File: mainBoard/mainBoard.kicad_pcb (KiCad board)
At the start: 4 copper layers, 50 x 60 mm, 46 parts, among them J1 Conn_01x04, J10 Conn_02x07_Odd_Even, J2 Conn_01x04, J3 Conn_01x03, J6 Conn_01x07, J7 Conn_01x07, J8 Conn_01x02, M1 Conn_01x01, M2 Conn_01x01, U1 MAX15062A, U2 STM32H503CBT6, U3 DRV8251ADDAR

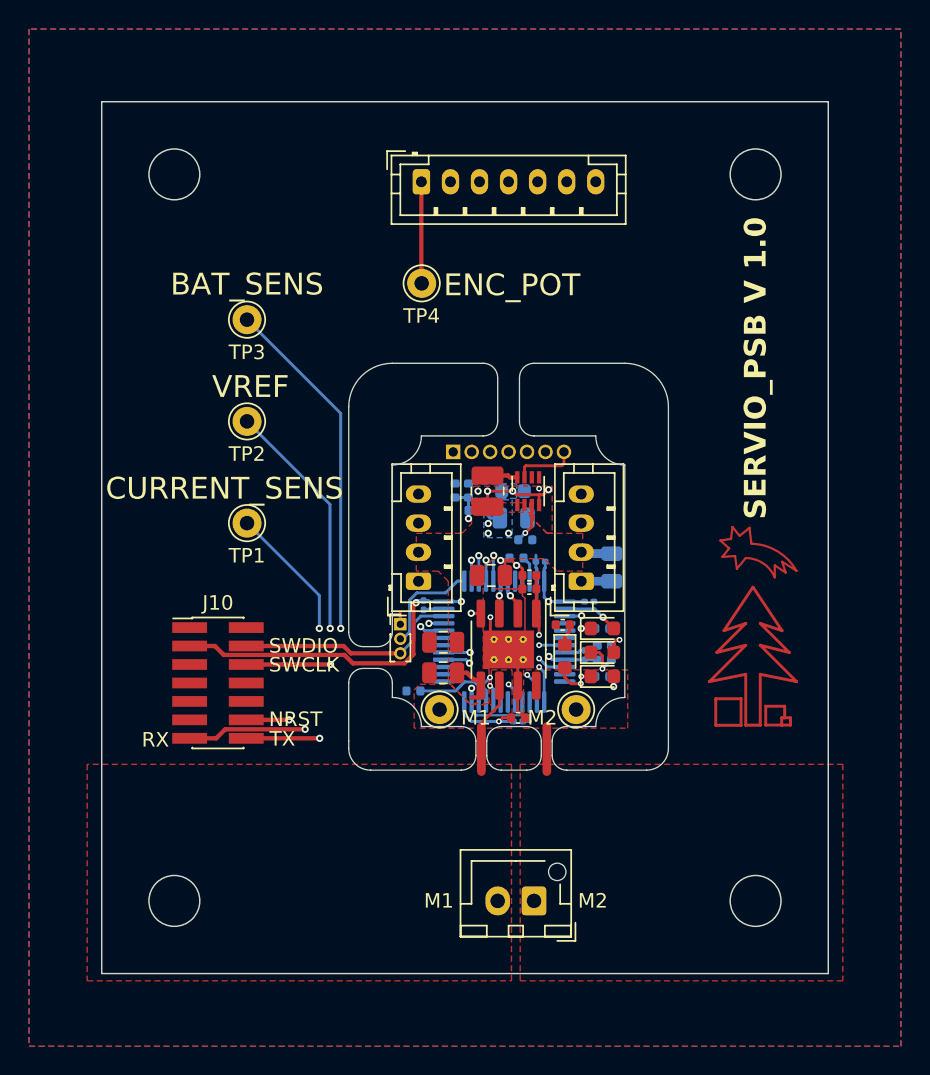
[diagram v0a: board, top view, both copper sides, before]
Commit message: drobeček
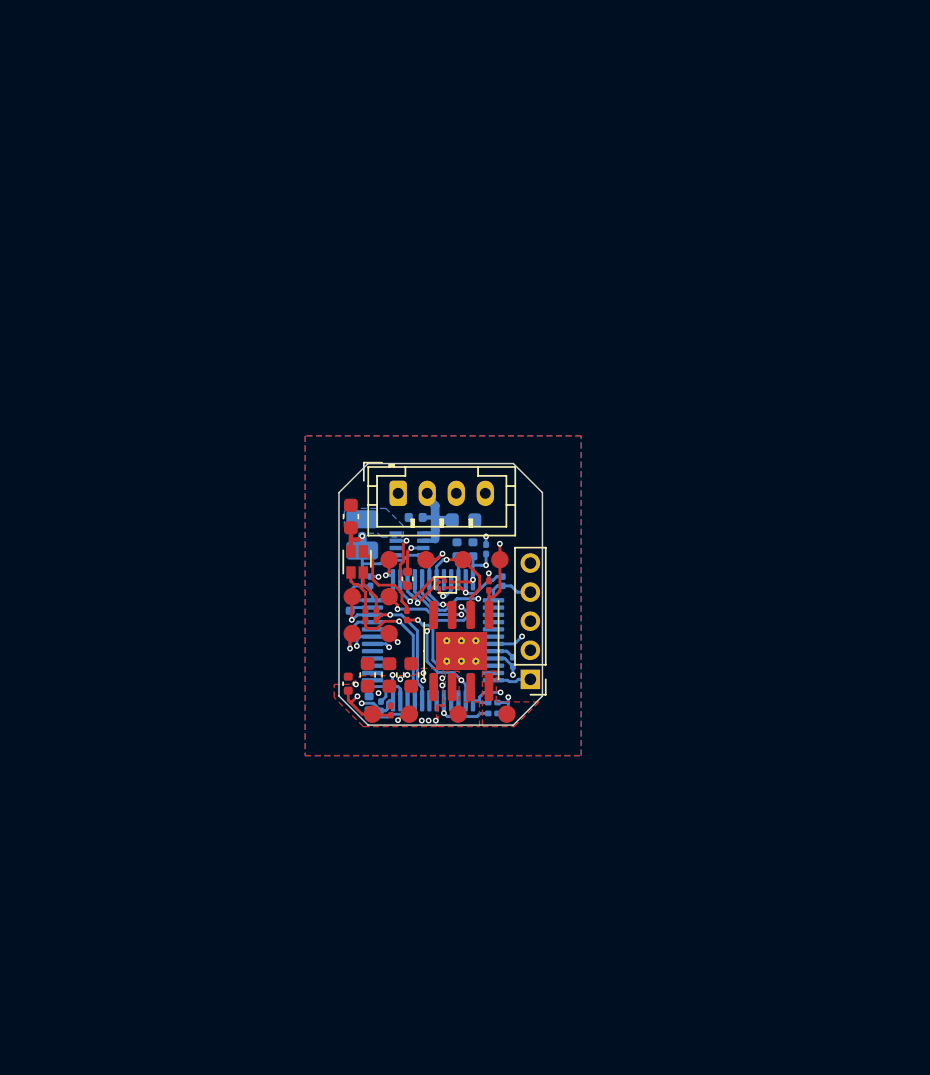
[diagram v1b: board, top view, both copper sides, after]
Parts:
- removed D1: LED-R, LED_SMD:LED_0603_1608Metric
- removed D2: LED-G, LED_SMD:LED_0603_1608Metric
- removed D3: LED-B, LED_SMD:LED_0603_1608Metric
- removed D4: LED-Y, LED_SMD:LED_0603_1608Metric
- removed R3: 1k, Capacitor_SMD:C_0402_1005Metric
- removed TP1, TP2, TP3, TP4: Conn_01x01, Connector_Pin:Pin_D1.0mm_L10.0mm
- added D5: LED_RGAB, LED_SMD:LED_LiteOn_LTST-C19HE1WT, F.Cu at (142.6, 96.7)
- added J11: Conn_01x01, RKL-Connectors:YZ157015035P-01-contact_pad, F.Cu at (144.8, 99.1)
- added J12: Conn_01x01, RKL-Connectors:YZ157015035P-01-contact_pad, F.Cu at (142.2, 101.6)
- added J13: Conn_01x01, RKL-Connectors:YZ157015035P-01-contact_pad, F.Cu at (144.8, 101.6)
- added J4: Conn_01x01, RKL-Connectors:YZ157015035P-01-contact_pad, F.Cu at (146.2, 107.2)
- added J9: Conn_01x01, RKL-Connectors:YZ157015035P-01-contact_pad, F.Cu at (142.2, 99.1)
- added U4: 64Kbit, RKL-StandardPackages:XFBGA-6, F.Cu at (148.7, 98.2)
- C1, C3, C4: moved to F.Cu
- C14: footprint Capacitor_SMD:C_0805_2012Metric -> Capacitor_SMD:C_0603_1608Metric; moved to F.Cu
- C15, R6: footprint Capacitor_SMD:C_0402_1005Metric -> Capacitor_SMD:C_0201_0603Metric
- C16, C17: footprint Capacitor_SMD:C_0805_2012Metric -> Capacitor_SMD:C_0603_1608Metric
- C18: footprint Capacitor_SMD:C_0805_2012Metric -> Capacitor_SMD:C_0603_1608Metric; moved to B.Cu
- C2: footprint Capacitor_SMD:C_0805_2012Metric -> Capacitor_SMD:C_0402_1005Metric
- C5, L1, U1: moved to B.Cu
- J10: value Conn_02x07_Odd_Even -> Conn_01x01; footprint Connector_PinHeader_1.27mm:PinHeader_2x07_P1.27mm_Vertical_SMD -> RKL-Connectors:YZ157015035P-01-contact_pad
- J2: value Conn_01x04 -> Conn_01x01; footprint Connector_JST:JST_PH_B4B-PH-K_1x04_P2.00mm_Vertical -> RKL-Connectors:YZ157015035P-01-contact_pad
- J3: value Conn_01x03 -> Conn_01x01; footprint Connector_PinHeader_1.00mm:PinHeader_1x03_P1.00mm_Vertical -> RKL-Connectors:YZ157015035P-01-contact_pad
- J6: value Conn_01x07 -> Conn_01x01; footprint Connector_JST:JST_PH_B7B-PH-K_1x07_P2.00mm_Vertical -> RKL-Connectors:YZ157015035P-01-contact_pad
- J7: value Conn_01x07 -> Conn_01x05; footprint Connector_PinHeader_1.27mm:PinHeader_1x07_P1.27mm_Vertical -> Connector_PinHeader_2.00mm:PinHeader_1x05_P2.00mm_Vertical; moved to F.Cu
- J8: value Conn_01x02 -> Conn_01x01; footprint Connector_JST:JST_XH_B2B-XH-AM_1x02_P2.50mm_Vertical -> RKL-Connectors:YZ157015035P-01-contact_pad
- M1, M2: footprint Connector_Pin:Pin_D1.0mm_L10.0mm -> RKL-Connectors:YZ157015035P-01-contact_pad
- R1: footprint Capacitor_SMD:C_0402_1005Metric -> Resistor_SMD:R_0201_0603Metric; moved to F.Cu
- R2: footprint Capacitor_SMD:C_0402_1005Metric -> Resistor_SMD:R_0201_0603Metric
- R4, R5: footprint Capacitor_SMD:C_0402_1005Metric -> Capacitor_SMD:C_0201_0603Metric; moved to F.Cu
- R7: footprint Capacitor_SMD:C_0402_1005Metric -> Capacitor_SMD:C_0201_0603Metric; moved to B.Cu
- moved J6 26.0 mm to (147.3, 96.5)
- moved J8 24.0 mm to (149.9, 96.5), turned to 0 degrees
- moved J2 17.0 mm to (143.6, 107.2), turned to 0 degrees
- moved R4 16.8 mm to (143.2, 100.3), turned to -90 degrees
- moved J7 16.5 mm to (154.5, 104.8), turned to 180 degrees
- moved R5 16.4 mm to (143.9, 100.3), turned to -90 degrees
- moved C14 15.7 mm to (146.3, 104.5), turned to 90 degrees
- moved C1 15.7 mm to (142.0, 105.0)
- moved R2 15.6 mm to (151.9, 107.1), turned to 180 degrees
- moved C6 15.1 mm to (143.5, 98.0), turned to 90 degrees
- moved R1 14.9 mm to (144.9, 106.9), turned to -90 degrees
- moved J10 14.5 mm to (144.8, 96.5)
- moved C10 14.5 mm to (144.2, 106.6)
- moved C5 14.0 mm to (142.1, 99.5), turned to -90 degrees
- moved C7 12.1 mm to (151.4, 95.8), turned to 90 degrees
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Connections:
- J10 pad 1: unconnected-(J10-Pin_1-Pad1) -> /CPU/SWCLK
- J2 pad 1: GND -> /CPU/MEŘENÍ-NAPÁJENÍ
- J3 pad 1: GND -> /CPU/DRV.PROUD
- J6 pad 1: /CPU/ENC.POT -> /CPU/DRV.IN1
- J7 pad 1: /CPU/ENC.POT -> /CPU/ENC.CLK
- J7 pad 2: /CPU/ENC.ENC-TYP-DET -> /CPU/ENC.MISO
- J7 pad 3: /CPU/ENC.CLK -> /CPU/ENC.MOSI
- J7 pad 4: /CPU/ENC.MISO -> VDD
- J7 pad 5: /CPU/ENC.MOSI -> GND
- J8 pad 1: Net-(J8-Pin_1) -> /CPU/DRV.IN2
- M1 pad 1: Net-(J8-Pin_2) -> Net-(M1-Pin_1)
- M2 pad 1: Net-(J8-Pin_1) -> Net-(M2-Pin_1)
- R4 pad 2: GND -> /CPU/LED.G
- R5 pad 2: GND -> /CPU/LED.R
- R6 pad 2: GND -> /CPU/LED.B
- U2 pad 10: /CPU/ENC.POT -> /CPU/LED.B
- U2 pad 12: unconnected-(U2-PA2-Pad12) -> /CPU/ENC.CLK
- U2 pad 2: /CPU/LED.R -> unconnected-(U2-PC13-Pad2)
- U2 pad 20: /CPU/LED.G -> /CPU/LED.R
- U2 pad 21: /CPU/LED.Y -> /CPU/LED.G
- U2 pad 28: /CPU/UART.RX -> unconnected-(U2-PB15-Pad28)
- U2 pad 29: /CPU/UART.TX -> unconnected-(U2-PA8-Pad29)
- U2 pad 3: /CPU/LED.B -> unconnected-(U2-PC14-_OSC32_IN(OSC32_IN)-Pad3)
- U2 pad 30: unconnected-(U2-PA9-Pad30) -> /CPU/UART.TX
- U2 pad 31: unconnected-(U2-PA10-Pad31) -> /CPU/UART.RX
- U2 pad 32: /CPU/RX-1 -> /CPU/RX-2
- U2 pad 33: /CPU/TX-1 -> /CPU/TX-2
- U2 pad 38: /CPU/ENC.ENC-TYP-DET -> /CPU/EEPROM.WP
- U2 pad 39: /CPU/ENC.CLK -> /CPU/EEPROM.SCL
- U2 pad 45: unconnected-(U2-PB8-Pad45) -> /CPU/EEPROM.SDA
- U3 pad 6: Net-(J8-Pin_2) -> Net-(M1-Pin_1)
- U3 pad 8: Net-(J8-Pin_1) -> Net-(M2-Pin_1)
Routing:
- net /CPU/ENC.POT: track 45.6 -> 0.00 mm, vias 2 -> 0
- net GND: track 62.2 -> 22.9 mm, vias 4 -> 7
- net /CPU/MEŘENÍ-NAPÁJENÍ: track 54.2 -> 15.2 mm, vias 3 -> 2
- net /CPU/ENC.ENC-TYP-DET: track 30.6 -> 0.00 mm, vias 1 -> 0
- net /CPU/DRV.VREF: track 42.3 -> 15.5 mm
- net /CPU/ENC.CLK: track 29.4 -> 2.64 mm, vias 1 -> 0
- net /CPU/RX-1: track 23.1 -> 0.00 mm, vias 2 -> 0
- net /CPU/TX-1: track 19.9 -> 0.00 mm, vias 2 -> 0
- net /CPU/ENC.MOSI: track 29.7 -> 9.83 mm
- net VDD: track 92.6 -> 72.9 mm, vias 9 -> 5
- net /CPU/ENC.MISO: track 28.1 -> 10.4 mm
- net /CPU/DRV.PROUD: track 37.3 -> 20.5 mm, vias 3 -> 2
- net /CPU/SWCLK: track 18.7 -> 1.98 mm
- net /CPU/NRST: track 29.2 -> 14.5 mm, vias 2 -> 3
- net /CPU/SWDIO: track 15.5 -> 3.18 mm, vias 0 -> 1
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- added copper zone on F.Cu, net Net-(M1-Pin_1)
- added copper zone on F.Cu, net Net-(M2-Pin_1)
- added copper zone on B.Cu, net Net-(U1-LX)
- added copper zone on In2.Cu, net VCC
- added copper zone on In2.Cu, net VDD
- removed copper zone on In2.Cu, net GND
- removed copper zone on F.Cu, net Net-(J8-Pin_1)
- removed copper zone on F.Cu, net Net-(J8-Pin_2)
- removed copper zone on B.Cu, net VCC
- removed copper zone on B.Cu, net VDD
- removed copper zone on F.Cu, net VDD
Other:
- board size 50 x 60 mm -> 14 x 18 mm
- board text removed: "+"
- board text removed: "-"
- board text removed: "BAT_SENS"
- board text removed: "CLK"
- board text removed: "CURRENT_SENS"
- board text removed: "E.TYP"
- board text removed: "ENC_POT"
- board text removed: "M1"
- board text removed: "M2"
- board text removed: "MISO"
- board text removed: "MOSI"
- board text removed: "NRST"
- board text removed: "POT"
- board text removed: "RX"
- board text removed: "SERVIO_PSB V 1.0"
- board text removed: "SWCLK"
- board text removed: "SWDIO"
- board text removed: "TX"
- board text removed: "VREF"
